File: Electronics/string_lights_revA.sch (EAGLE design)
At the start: 25 parts, among them U1 ESP32-ADAPTER

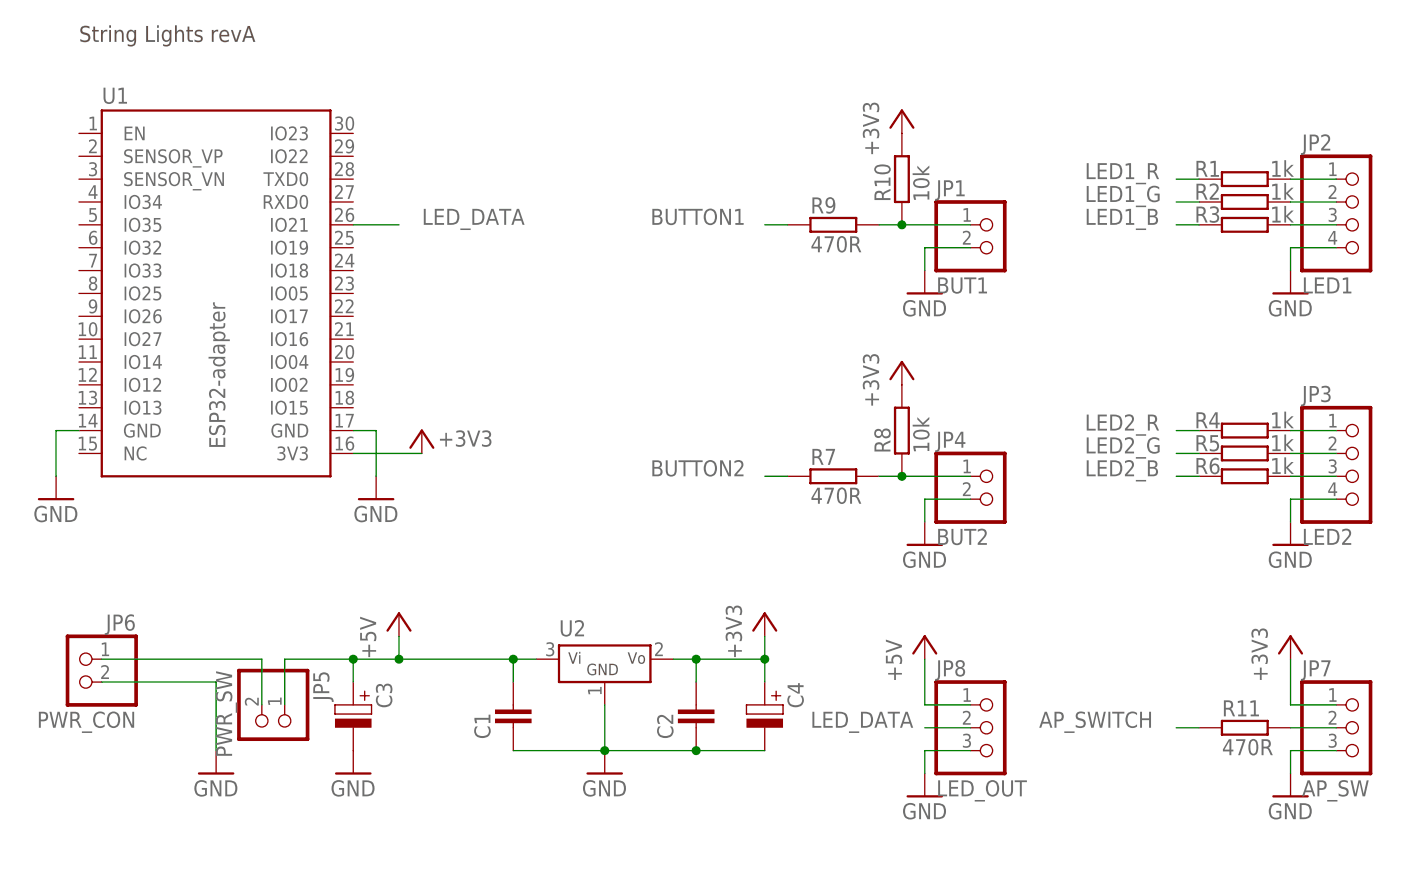
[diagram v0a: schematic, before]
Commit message: Electronics: finished RevA
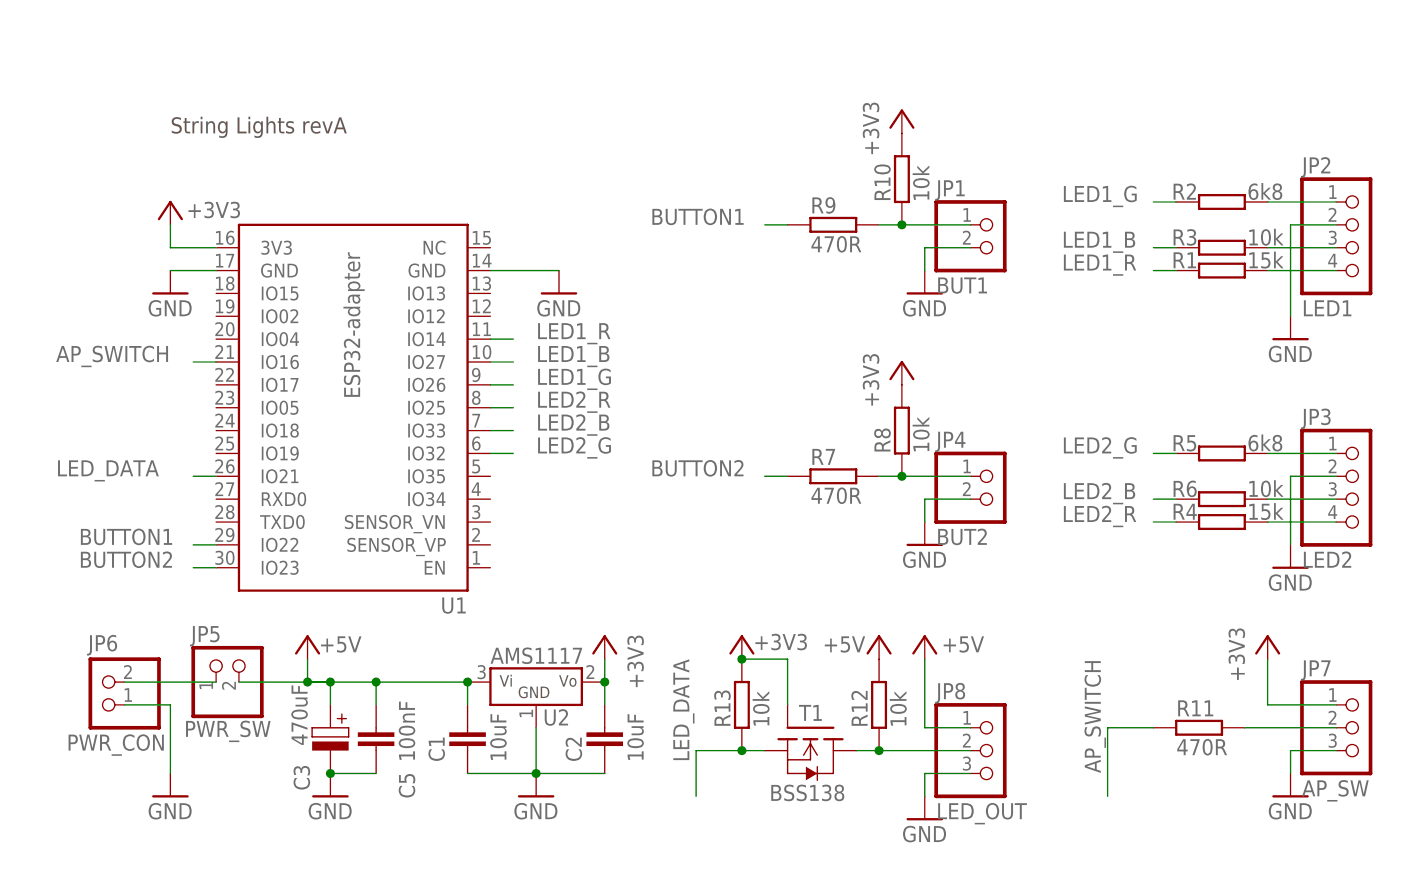
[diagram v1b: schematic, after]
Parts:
- removed C4: (no value), 1_domaci:C-POLY'10MM'
- added C5: 100nF, 1_domaci:C-CERAMIC'SMD'
- added R12, R13: 10k, 1_domaci:R'2'
- added T1: BSS138, 1_domaci:BSS138
- C1, C2: value (none) -> 10uF
- C3: value (none) -> 470uF
- R1, R4: value 1k -> 15k
- R2, R5: value 1k -> 6k8
- R3, R6: value 1k -> 10k
- U2: value (none) -> AMS1117
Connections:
- removed net N$3 (its old number): JP2.2, R2.P$2
- removed net N$6 (its old number): JP3.2, R5.P$2
- new net N$12: JP8.2, R12.P$1, T1.D
- new net N$4: JP2.1, R2.P$2
- new net N$7: JP3.4, R4.P$2
- net +3V3: now also R13.P$2, T1.G; no longer C4.POS
- net +5V: now also C5.P$2, JP5.2, R12.P$2; no longer JP5.1
- net AP_SWITCH: now also U1.IO16
- net BUTTON1: now also U1.IO22
- net BUTTON2: now also U1.IO23
- net GND: now also C5.P$1, JP2.2, JP3.2, JP6.1; no longer C4.NEG, JP2.4, JP3.4, JP6.2
- net LED1_B: now also U1.IO27
- net LED1_G: now also U1.IO26
- net LED1_R: now also U1.IO14
- net LED2_B: now also U1.IO33
- net LED2_G: now also U1.IO32
- net LED2_R: now also U1.IO25
- net LED_DATA: now also R13.P$1, T1.S; no longer JP8.2
- net N$1: now also JP5.1, JP6.2; no longer JP5.2, JP6.1
- net N$2: now also JP2.4; no longer JP2.1
- net N$5: now also R5.P$2; no longer R4.P$2
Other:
- moved on the sheet: C1, C2, C3, JP2, JP3, JP5, JP6, JP8, R1, R11, R2, R3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
